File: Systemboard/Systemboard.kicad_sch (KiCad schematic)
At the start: 9 parts, among them J1 Conn_01x60, J108 Prog BT, U101 ESP32-WROOM-32E

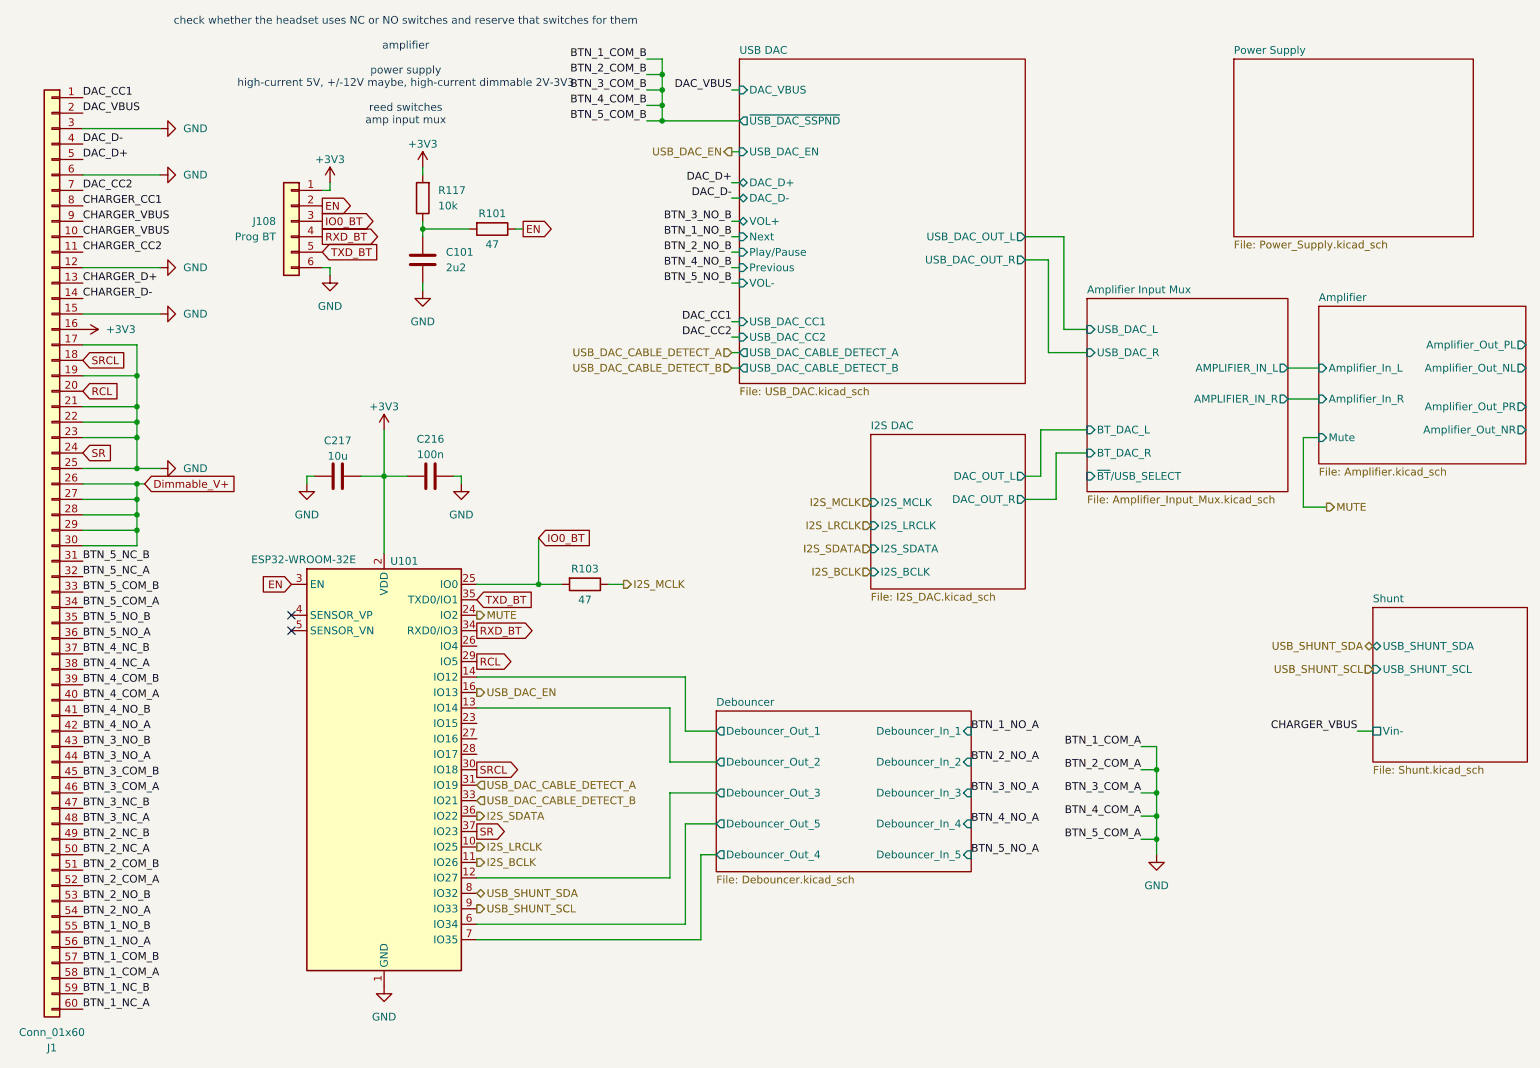
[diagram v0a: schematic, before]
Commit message: user save
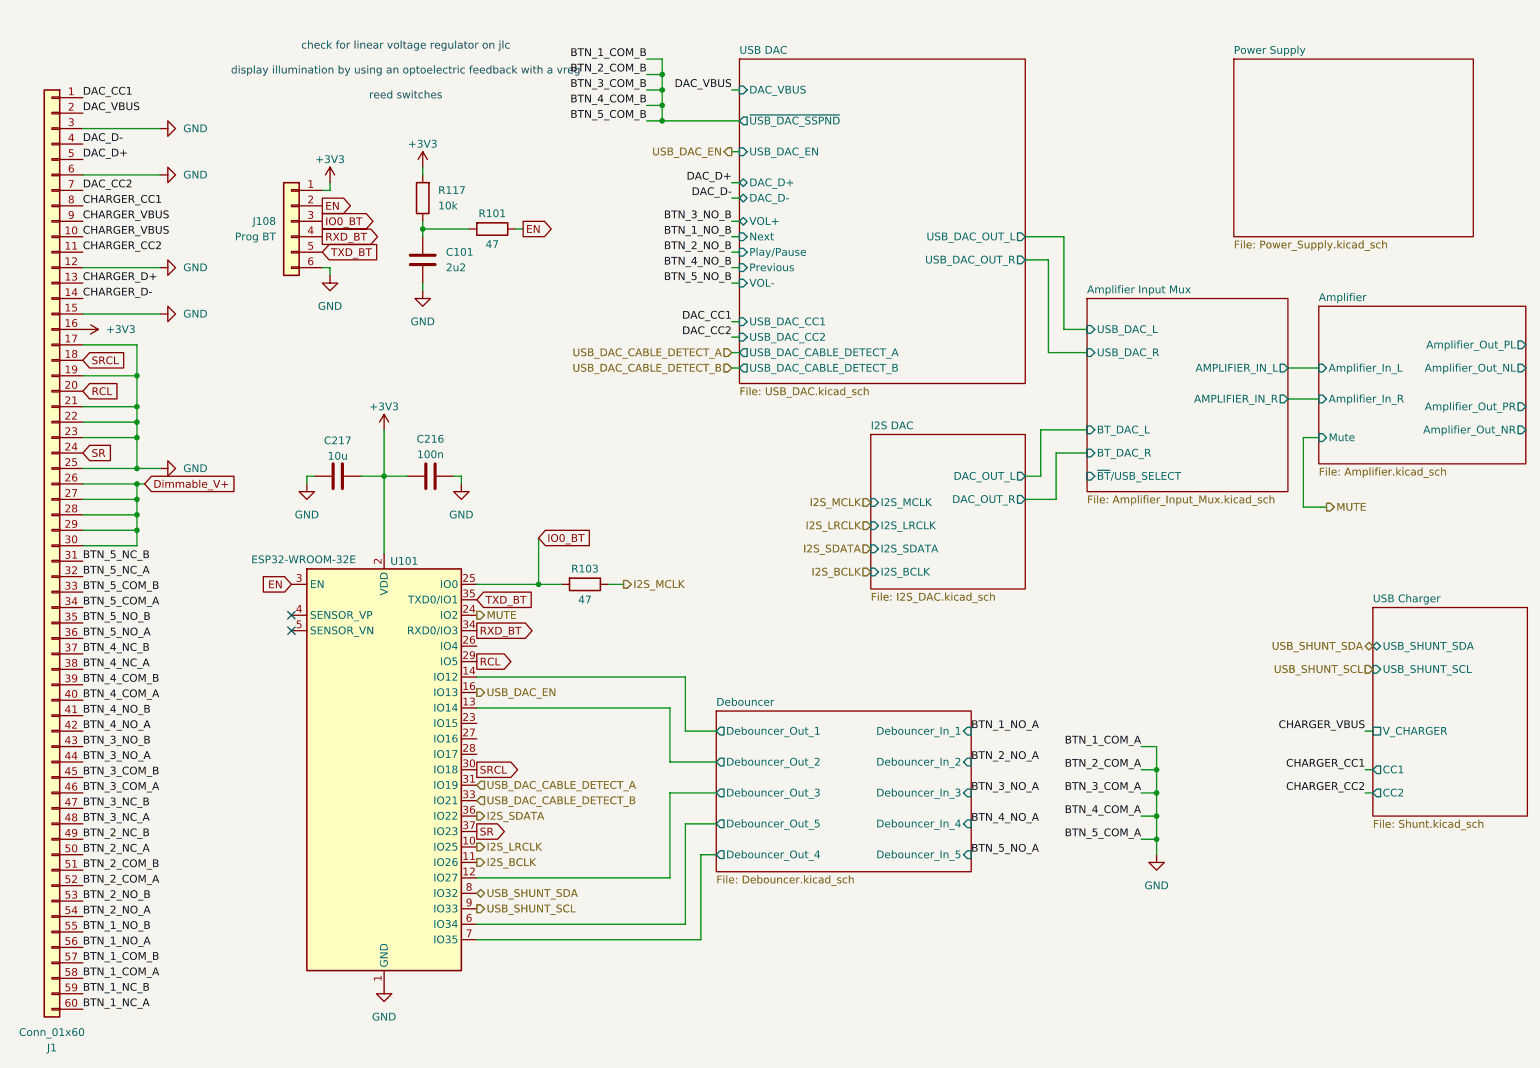
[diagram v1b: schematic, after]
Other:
- sheet Shunt renamed USB Charger
- sheet USB Charger ports: added CC1, CC2, V_CHARGER; removed Vin-
- note added: "check for linear voltage regulator on jlc display illumination by using an optoelectric feedback with a vreg reed switches"
- note removed: "check whether the headset uses NC or NO switches and reserve that switches for them amplifier power supply high-current 5V, +/-12V maybe, high-current dimmable 2V-3V3 reed switches amp input mux"
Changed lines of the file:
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@@
 	(generator_version "10.0")
 	(paper "A4")
-	(text "check whether the headset uses NC or NO switches and reserve that switches for them\n\namplifier\n\npower supply\nhigh-current 5V, +/-12V maybe, high-current dimmable 2V-3V3\n\nreed switches\namp input mux"
+	(text "check for linear voltage regulator on jlc\n\ndisplay illumination by using an optoelectric feedback with a vreg\n\nreed switches"
 		(exclude_from_sim no)
 		(at 84.836 22.352 0)
@@
 	(wire
 		(pts
-			(xy 241.3 130.81) (xy 243.84 130.81)
+			(xy 208.28 144.78) (xy 205.74 144.78)
 		)
 		(stroke
@@
 	(wire
 		(pts
-			(xy 208.28 144.78) (xy 205.74 144.78)
+			(xy 138.43 66.04) (xy 139.7 66.04)
 		)
 		(stroke
@@
 	(wire
 		(pts
-			(xy 138.43 66.04) (xy 139.7 66.04)
+			(xy 193.04 64.77) (xy 196.85 64.77)
 		)
 		(stroke
@@
 	(wire
 		(pts
-			(xy 193.04 64.77) (xy 196.85 64.77)
+			(xy 96.52 162.56) (xy 130.81 162.56)
 		)
 		(stroke
@@
 	(wire
 		(pts
-			(xy 96.52 162.56) (xy 130.81 162.56)
+			(xy 31.75 77.47) (xy 40.64 77.47)
 		)
 		(stroke
@@
 	(wire
 		(pts
-			(xy 31.75 77.47) (xy 40.64 77.47)
+			(xy 242.57 140.97) (xy 243.84 140.97)
 		)
 		(stroke
@@
 	(wire
 		(pts
+			(xy 242.57 137.16) (xy 243.84 137.16)
+		)
+		(stroke
+			(width 0)
+			(type default)
+		)
+	)
+	(wire
+		(pts
 			(xy 186.69 92.71) (xy 191.77 92.71)
 		)
@@
 		)
 	)
+	(wire
+		(pts
+			(xy 242.57 130.81) (xy 243.84 130.81)
+		)
+		(stroke
+			(width 0)
+			(type default)
+		)
+	)
 	(label "BTN_1_COM_B"
 		(at 124.46 20.32 180)
@@
 		)
 	)
+	(label "CHARGER_CC2"
+		(at 242.57 140.97 180)
+		(effects
+			(font
+				(size 1.27 1.27)
+			)
+			(justify right bottom)
+		)
+	)
 	(label "CHARGER_D-"
 		(at 31.75 59.69 0)
@@
 	)
 	(label "CHARGER_VBUS"
-		(at 241.3 130.81 180)
+		(at 242.57 130.81 180)
 		(effects
 			(font
@@
 		)
 	)
+	(label "CHARGER_CC1"
+		(at 242.57 137.16 180)
+		(effects
+			(font
+				(size 1.27 1.27)
+			)
+			(justify right bottom)
+		)
+	)
 	(label "DAC_CC1"
 		(at 31.75 26.67 0)
@@
 	(sheet
 		(at 243.84 110.49)
-		(size 25.4 25.4)
+		(size 25.4 34.29)
 		(exclude_from_sim no)
 		(in_bom yes)
@@
 			(color 0 0 0 0)
 		)
-		(property "Sheetname" "Shunt"
+		(property "Sheetname" "USB Charger"
 			(at 243.84 109.7784 0)
 			(show_name no)
@@
 		)
 		(property "Sheetfile" "Shunt.kicad_sch"
-			(at 243.84 136.4746 0)
+			(at 243.84 145.3646 0)
 			(show_name no)
 			(do_not_autoplace no)
@@
 			)
 		)
-		(pin "Vin-" passive
+		(pin "V_CHARGER" passive
 			(at 243.84 130.81 180)
 			(effects
 				(font
+					(size 1.27 1.27)
+				)
+				(justify left)
+			)
+		)
+		(pin "CC2" output
+			(at 243.84 140.97 180)
+			(effects
+				(font
+					(size 1.27 1.27)
+				)
+				(justify left)
+			)
+		)
+		(pin "CC1" output
+			(at 243.84 137.16 180)
+			(effects
+				(font
